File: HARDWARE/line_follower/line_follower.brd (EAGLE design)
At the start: 67.3 x 88.9 mm, 70 parts, among them IC1 L3GD20HSMD, IC2 L6205, IC3 ATMEGA328PMA, IC4 LF33, J1 FFC2B05-10-X_REVC, J2 FFC2B05-10-X_REVC, Q1 10MHz, T1 ELPT15-21C, T2 ELPT15-21C, T3 ELPT15-21C, T4 ELPT15-21C, T5 ELPT15-21C, T6 ELPT15-21C, X1 MINI-USB-SCHIELD-32005-201

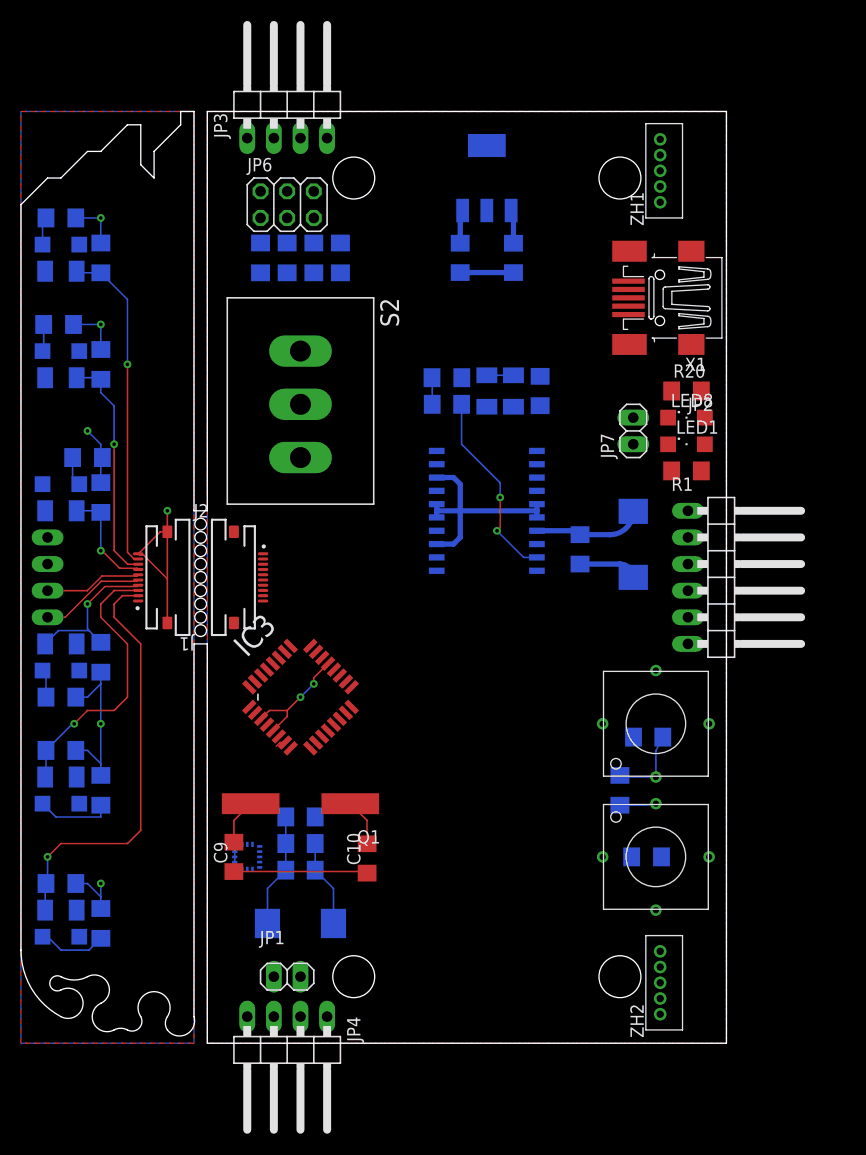
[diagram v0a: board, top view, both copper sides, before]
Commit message: finished PCB
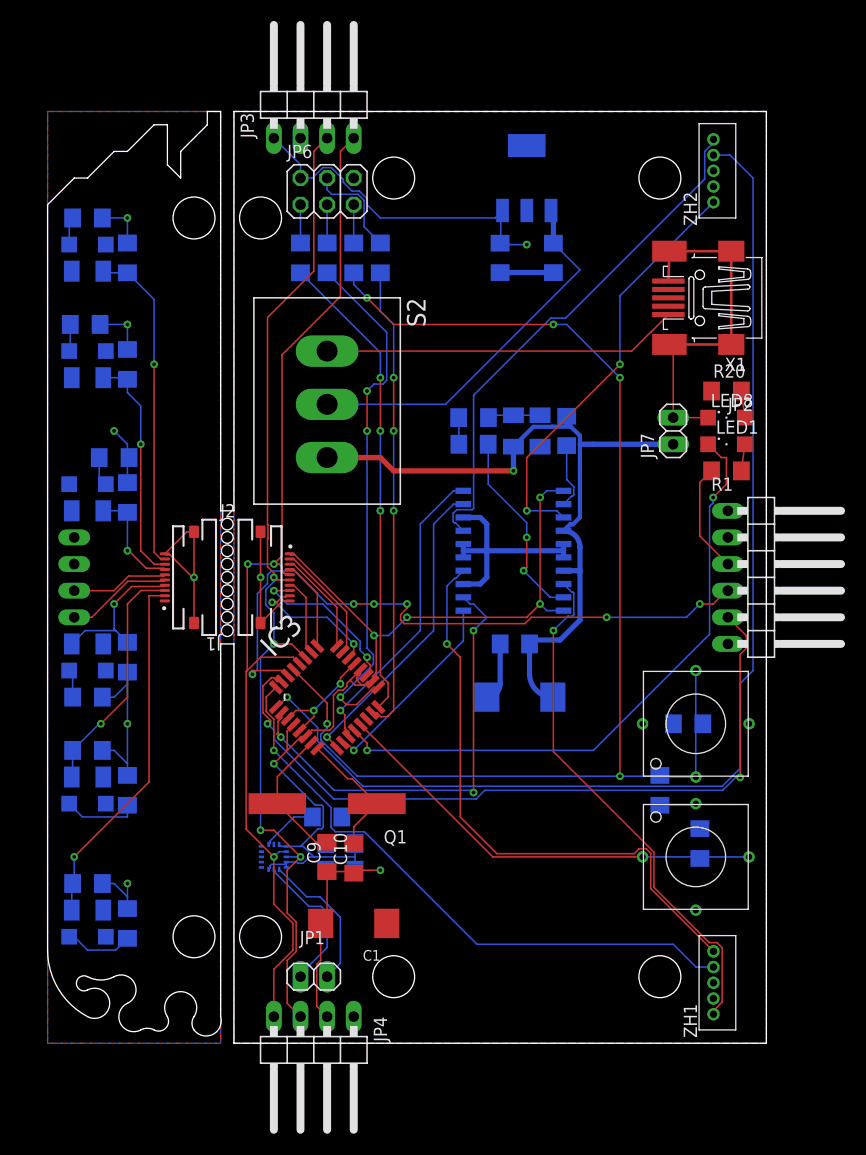
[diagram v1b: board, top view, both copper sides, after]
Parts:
- moved ZH1 77.6 mm to (62.2, 1.27)
- moved ZH2 77.6 mm to (62.2, 78.7)
- moved C5 18.2 mm to (45.1, 33.0), turned to 0 degrees
- moved C6 11.0 mm to (44.6, 38.1), turned to 0 degrees
- moved C9 8.89 mm to (26.7, 17.8)
- moved R2 5.24 mm to (62.2, 19.1), turned to 90 degrees
- moved C1 5.08 mm to (29.2, 11.4), flipped to the top, turned to 180 degrees
- moved C8 4.58 mm to (40.6, 57.1)
- moved R3 4.58 mm to (40.6, 59.7)
- moved D1 4.58 mm to (44.5, 58.4)
- moved IC2 4.58 mm to (44.5, 47.0)
- moved C7 4.58 mm to (49.5, 58.4)
- moved D2 4.58 mm to (47.0, 58.4)
- moved C13 4.02 mm to (61.1, 30.5)
- moved JP6 4.02 mm to (26.7, 81.3)
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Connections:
- new net N$10: C11.1, IC4.1, S2.COM
- net VB: no longer C11.1, IC4.1, S2.COM
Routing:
- net VCC: track 15.0 -> 143.7 mm, vias 0 -> 6
- net !RESET: track 7.46 -> 124.6 mm, vias 0 -> 5
- net INT1: track 0.14 -> 111.8 mm, vias 0 -> 1
- net SCL: track 0.00 -> 101.5 mm, vias 0 -> 3
- net SDA: track 0.00 -> 98.2 mm, vias 0 -> 4
- net TX: track 0.00 -> 72.1 mm, vias 0 -> 2
- net RX: track 0.00 -> 63.9 mm, vias 0 -> 6
- net LED: track 0.00 -> 59.4 mm, vias 0 -> 2
- net INT0: track 0.00 -> 58.3 mm, vias 0 -> 1
- net VB: track 13.5 -> 70.5 mm, vias 0 -> 1
- net OUT1A: track 0.00 -> 56.6 mm, vias 0 -> 1
- net SCK: track 0.00 -> 50.4 mm, vias 0 -> 3
- net OUT2A: track 0.00 -> 50.0 mm, vias 0 -> 1
- net OUT1B: track 0.00 -> 49.8 mm
- net MISO: track 0.00 -> 45.3 mm, vias 0 -> 3
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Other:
- board size 67.3 x 88.9 mm -> 68.6 x 88.9 mm
